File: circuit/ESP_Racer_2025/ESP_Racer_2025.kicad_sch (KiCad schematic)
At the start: 19 parts, among them IC1 XCL102D333CR-G, J1 Conn_LED_1, J2 Conn_LED_2, J3 Conn_Servo, U1 DRV8835DSST, U2 SFV12R-2STE1LF, U3 ESP32-C3-WROOM-02

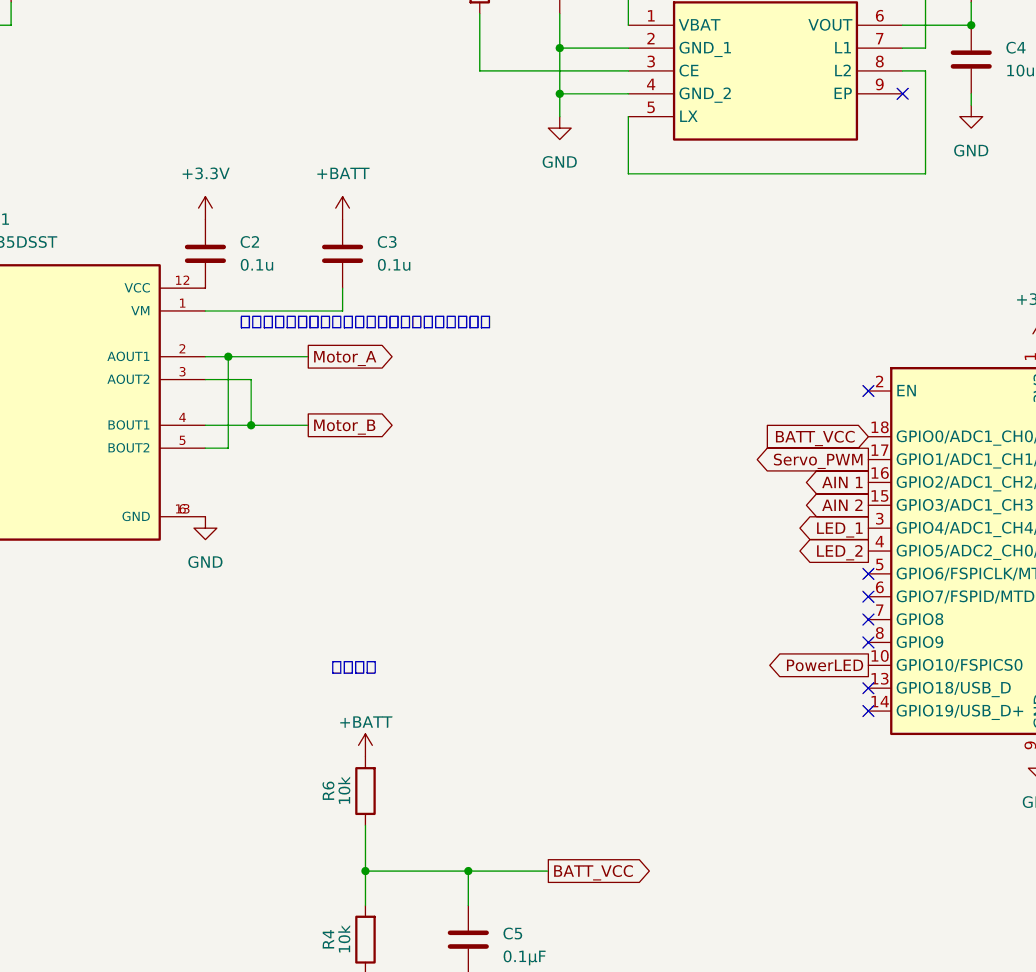
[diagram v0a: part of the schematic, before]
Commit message: pcb fix
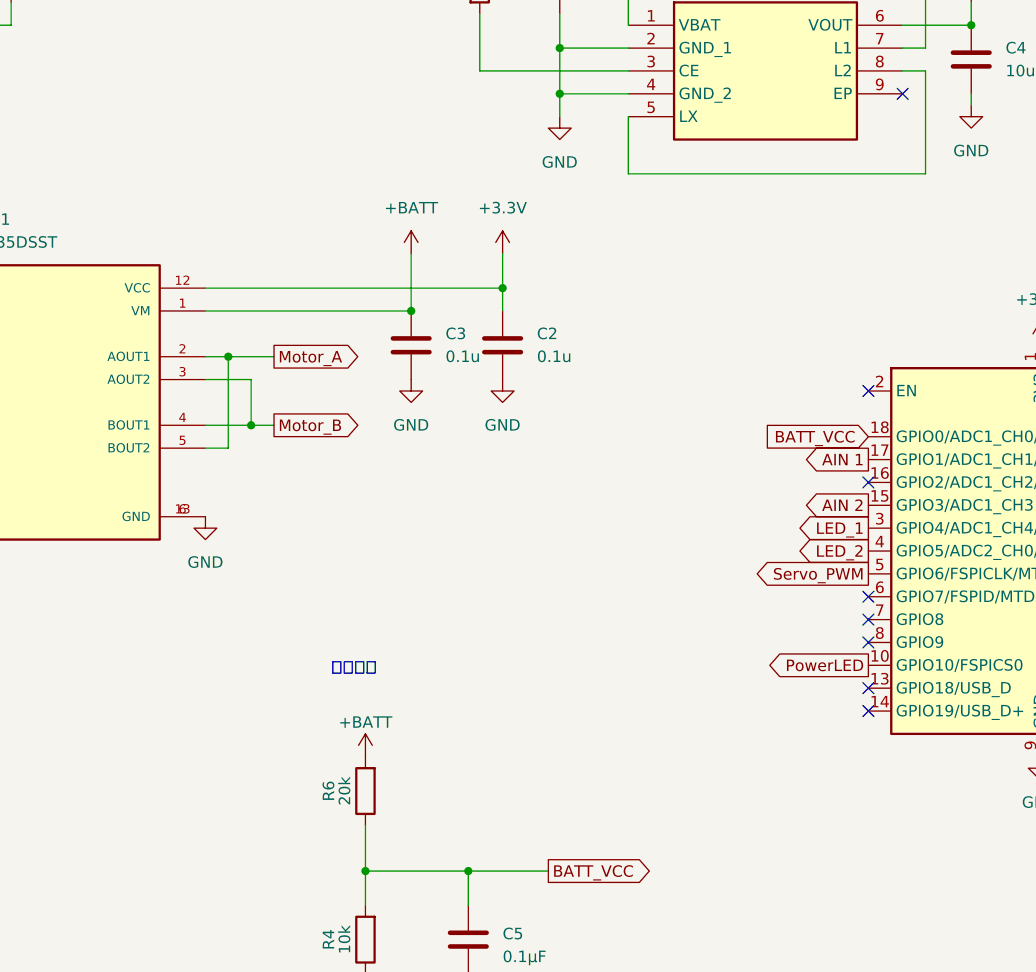
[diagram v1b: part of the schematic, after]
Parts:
- J1, J2: footprint JST_ZH_B2B-ZR_1x02_P1.50mm_Vertical:JST_ZH_B2B-ZR_1x02_P1.50mm_Vertical -> Molex:Molex_PicoBlade_53047-0210_1x02_P1.25mm_Vertical
- J3: footprint JST_ZH_B3B-ZR_1x03_P1.50mm_Vertical:JST_ZH_B3B-ZR_1x03_P1.50mm_Vertical -> Molex:Molex_PicoBlade_53047-0310_1x03_P1.25mm_Vertical
- R6: value 10k -> 20k
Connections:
- net +3.3V: now also U1.12 (VCC)
- net +BATT: now also U1.1 (VM)
- net AIN 1: now also U3.17 (GPIO1/ADC1_CH1/XTAL_N); no longer U3.16 (GPIO2/ADC1_CH2/FSPIQ)
- net GND: now also C2.2, C3.2
- net Servo_PWM: now also U3.5 (GPIO6/FSPICLK/MTCK); no longer U3.17 (GPIO1/ADC1_CH1/XTAL_N)
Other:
- note removed: "少しパターンを細長くして電流のピークを抑える"
- moved on the sheet: C2, C3
